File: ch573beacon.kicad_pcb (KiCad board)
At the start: 2 copper layers, 34 x 34 mm, 33 parts, among them J1 USB_C_Receptacle_USB2.0, SW1 SW_Push, U1 BH1750FVI, U2 ME6216A33M3G, U3 CH573F, U4 SHT31-DIS, U5 TP4054, Y1 Crystal, Y2 Crystal_GND24

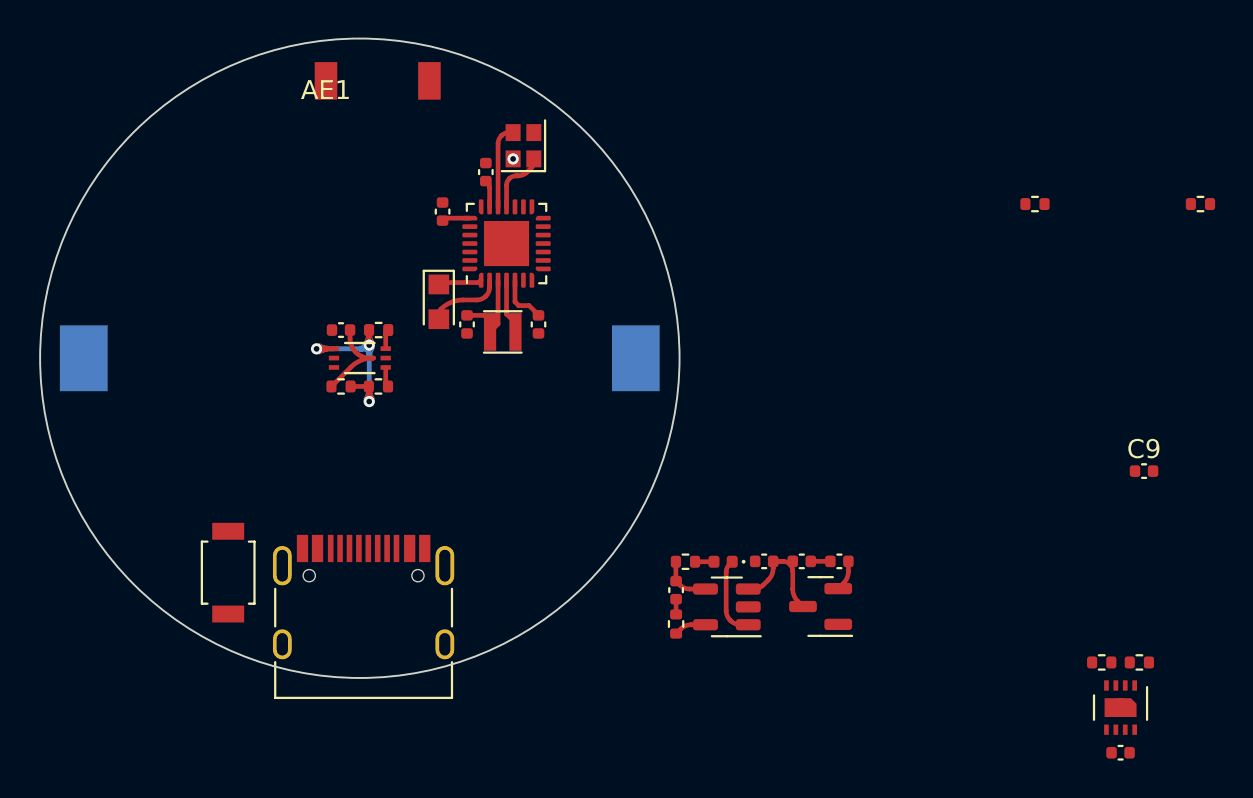
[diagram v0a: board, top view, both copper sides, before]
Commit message: update
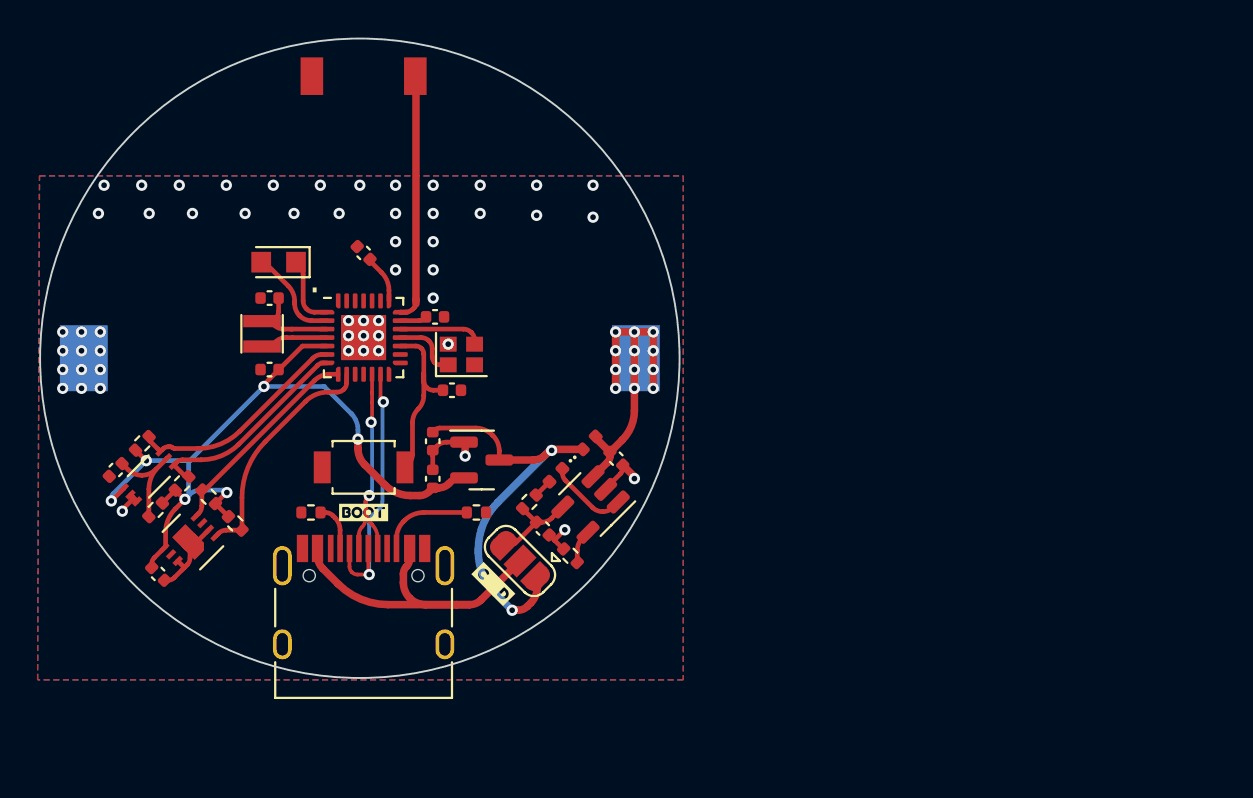
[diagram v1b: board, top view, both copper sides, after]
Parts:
- added D1: D, Diode_SMD:D_0402_1005Metric, F.Cu at (132.8, 130.7)
- added JP1: Jumper_3_Bridged12, Jumper:SolderJumper-3_P1.3mm_Open_RoundedPad1.0x1.5mm, F.Cu at (129.1, 137.0)
- added kibuzzard-64141A9C: G***, kibuzzard-64141A9C, F.Cu at (127.7, 138.2)
- added kibuzzard-64142EB1: G***, kibuzzard-64142EB1, F.Cu at (120.8, 134.4)
- AE1: value Antenna -> Antenna_Chip; footprint my:CA-C03 -> BLab:CA-03
- moved C8 52.1 mm to (109.9, 137.7), turned to -45 degrees
- moved U4 50.3 mm to (111.6, 136.0), turned to -135 degrees
- moved R4 48.6 mm to (114.0, 135.0), turned to -45 degrees
- moved R5 48.3 mm to (112.6, 133.6), turned to 135 degrees
- moved R7 41.8 mm to (126.8, 134.4), turned to 0 degrees
- moved R6 41.8 mm to (118.0, 134.4)
- moved C10 37.1 mm to (125.5, 127.9), turned to 180 degrees
- moved C4 22.1 mm to (124.5, 132.6), turned to 90 degrees
- moved U2 19.6 mm to (127.1, 131.6), turned to 0 degrees
- moved C3 18.7 mm to (124.5, 130.6), turned to -90 degrees
- moved C2 14.5 mm to (115.8, 126.8), turned to 0 degrees
- moved C5 14.1 mm to (107.6, 132.1), turned to -135 degrees
- moved R1 13.9 mm to (109.0, 130.7), turned to 45 degrees
- moved U1 12.9 mm to (109.4, 132.5), turned to 45 degrees
- moved L1 12.8 mm to (115.4, 124.9), turned to -90 degrees
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- renumbered C9 to C10, C10 to C11, C11 to C7, C7 to C8, C8 to C9, D1 to D2
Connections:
- AE1 pad 1: Net-(AE1-Pad1) -> unconnected-(AE1-Pad1)
- AE1 pad 2: (no net) -> Net-(AE1-Pad2)
- C3 pad 1: BAT -> DIRECT
- C9 pad 1: +5V -> CHARG
- R1 pad 1: +3V3 -> VCC
- R2 pad 1: +3V3 -> VCC
- R3 pad 1: +3V3 -> VCC
- R9 pad 1: +5V -> CHARG
- U1 pad 1: +3V3 -> VCC
- U2 pad 3: BAT -> DIRECT
- U3 pad 21: Net-(AE1-Pad1) -> Net-(AE1-Pad2)
- U3 pad 6: SDA_SHT -> SCL_BH
- U3 pad 7: SCL_SHT -> SDA_BH
- U3 pad 8: SCL_BH -> SCL_SHT
- U3 pad 9: SDA_BH -> SDA_SHT
- U5 pad 4: +5V -> CHARG
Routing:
- net VCC: track 4.37 -> 43.5 mm, vias 0 -> 6
- net DIRECT: track 0.00 -> 22.5 mm, vias 0 -> 2
- net +5V: track 2.74 -> 19.2 mm
- net D-: track 0.00 -> 14.6 mm, vias 0 -> 2
- net Net-(AE1-Pad2): track 0.00 -> 13.5 mm
- net BAT: track 5.49 -> 18.1 mm, vias 0 -> 12
- net SDA_SHT: track 0.00 -> 12.6 mm
- net D+: track 0.00 -> 12.5 mm, vias 0 -> 2
- net GND: track 1.85 -> 13.5 mm, vias 1 -> 54
- net SCL_SHT: track 0.00 -> 11.2 mm
- net SCL_BH: track 1.03 -> 11.8 mm
- net SDA_BH: track 1.05 -> 11.3 mm
- net BOOT: track 0.00 -> 9.49 mm
- net +3V3: track 9.37 -> 0.00 mm, vias 3 -> 0
- net CC2: track 0.00 -> 5.03 mm
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- added copper zone on B.Cu, net GND
- added copper zone on F.Cu, net GND
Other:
- board text added: "."

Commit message: update
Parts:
- C3, C4: value 4.7uf -> 0.1uf
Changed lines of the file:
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@@
       (effects (font (size 1 1) (thickness 0.15)))
     )
-    (fp_text value "4.7uf" (at 0 1.16 90) (layer "F.Fab")
+    (fp_text value "0.1uf" (at 0 1.16 90) (layer "F.Fab")
       (effects (font (size 1 1) (thickness 0.15)))
     )
@@
     (attr board_only exclude_from_pos_files exclude_from_bom)
     (fp_text reference "kibuzzard-64141A9C" (at 0 -3.511021 135) (layer "F.SilkS") hide
-      (effects (font (size 0 0)))
+      (effects (font (size 0 0) (thickness 0.15)))
     )
     (fp_text value "G***" (at 0 3.511021 135) (layer "F.SilkS") hide
-      (effects (font (size 0 0)))
+      (effects (font (size 0 0) (thickness 0.15)))
     )
     (fp_poly (pts
@@
     (attr board_only exclude_from_pos_files exclude_from_bom)
     (fp_text reference "kibuzzard-64142EB1" (at 0 -3.512608) (layer "F.SilkS") hide
-      (effects (font (size 0 0)))
+      (effects (font (size 0 0) (thickness 0.15)))
     )
     (fp_text value "G***" (at 0 3.512608) (layer "F.SilkS") hide
-      (effects (font (size 0 0)))
+      (effects (font (size 0 0) (thickness 0.15)))
     )
     (fp_poly (pts
@@
       (effects (font (size 1 1) (thickness 0.15)))
     )
-    (fp_text value "4.7uf" (at 0 1.16 90) (layer "F.Fab")
-      (effects (font (size 1 1) (thickness 0.15)))
-    )
+    (fp_text value "0.1uf" (at 0 1.16 90) (layer "F.Fab")
+      (effects (font (size 1 1) (thickness 0.15)))
+    )

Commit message: update
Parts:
- C9: value 4.7uf -> 1uf
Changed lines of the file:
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@@
       (effects (font (size 1 1) (thickness 0.15)))
     )
-    (fp_text value "4.7uf" (at 0 1.16 135) (layer "F.Fab")
+    (fp_text value "1uf" (at 0 1.16 135) (layer "F.Fab")
       (effects (font (size 1 1) (thickness 0.15)))
     )
